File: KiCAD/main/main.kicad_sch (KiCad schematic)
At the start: 42 parts, among them J1 USB_C_Receptacle_USB2.0_14P, J2 Conn_Coaxial, SW1 SW_SPDT, SW2 SW_Push, SW3 SW_Push, U1 SX1262IMLTRT, U2 TP4056-42-ESOP8, U3 TLV75533PDRV, U4 ESP32-S3-MINI-1, U5 BGS12WN6E6327

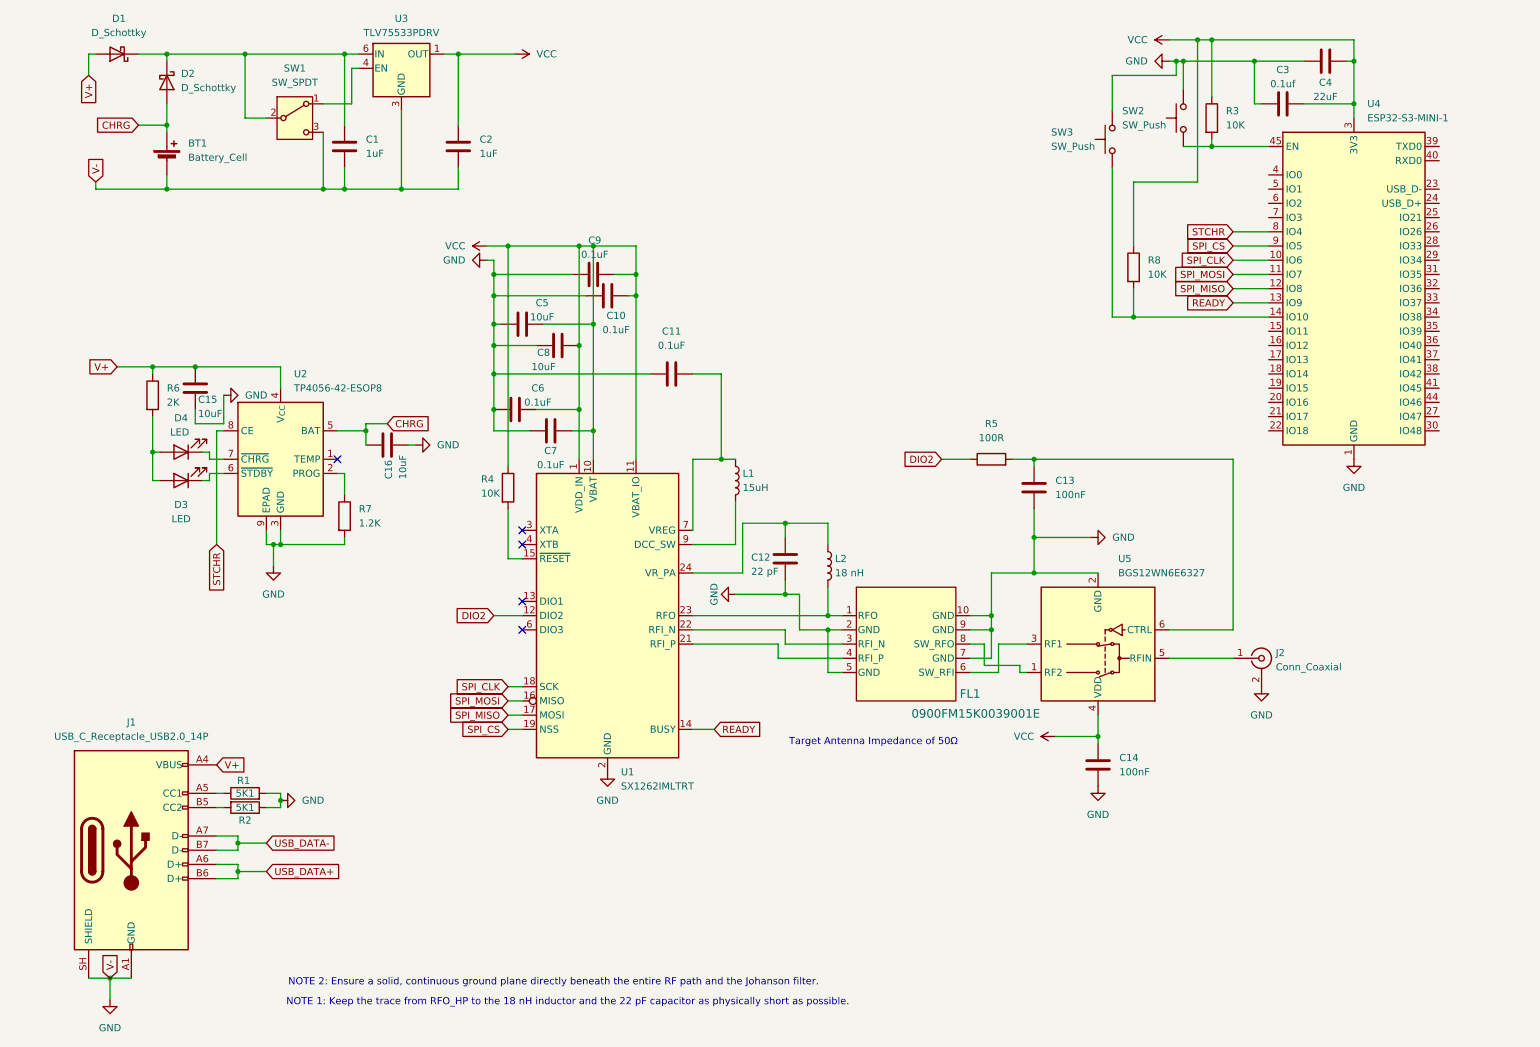
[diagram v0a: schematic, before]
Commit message: started repo and creation
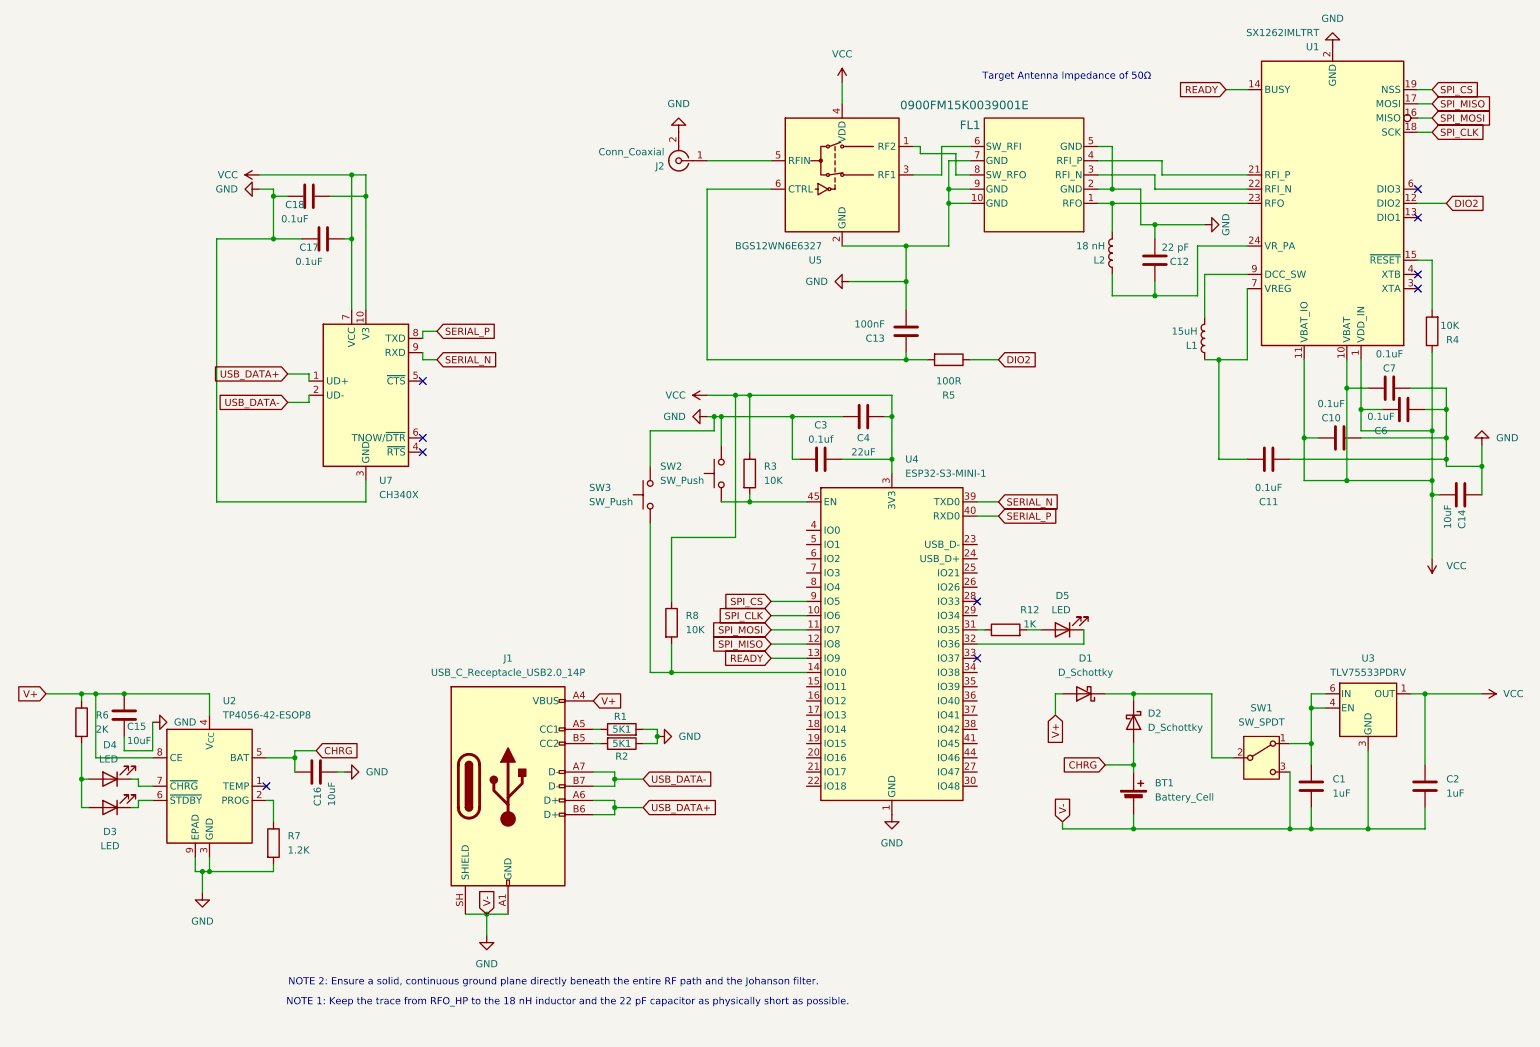
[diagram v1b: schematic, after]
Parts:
- removed C5, C8: 10uF, Capacitor_SMD:C_01005_0402Metric, symbol Device:C
- removed C9: 0.1uF, Capacitor_SMD:C_01005_0402Metric, symbol Device:C
- added C17, C18: 0.1uF, Capacitor_SMD:C_01005_0402Metric, symbol Device:C
- added D5: LED, LED_SMD:LED_0402_1005Metric, symbol Device:LED
- added R12: 1K, Resistor_SMD:R_01005_0402Metric, symbol Device:R
- added U7: CH340X, Package_SO:MSOP-10_3x3mm_P0.5mm, symbol Interface_USB:CH340X
- BT1: footprint Battery:BatteryHolder_MPD_BK-18650-PC2 -> Connector_JST:JST_PH_S2B-PH-K_1x02_P2.00mm_Horizontal
- C14: value 100nF -> 10uF
- R1, R2: footprint (none) -> Resistor_SMD:R_01005_0402Metric
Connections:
- net GND: now also C14.1, C17.1, C18.1, U7.3 (GND); no longer C14.2
- net USB_DATA+: now also U7.1 (UD+)
- net USB_DATA-: now also U7.2 (UD-)
- net V+: now also U2.8 (CE)
- net VCC: now also C14.2, C17.2, C18.2, U7.10 (V3), U7.7 (VCC); no longer C14.1
- net at U4.31 (IO35): now also R12.1
- net at U4.32 (IO36): now also D5.1 (K)
- net SERIAL_N: now reaches U4.39 (TXD0)
- net SERIAL_N: now also U7.9 (RXD)
- net SERIAL_P: now reaches U4.40 (RXD0)
- net SERIAL_P: now also U7.8 (TXD)
- net at D1.1 (K), D2.1 (K), SW1.2 (B): no longer C1.2, U3.6 (IN)
- net at SW1.1 (A), U3.4 (EN): now also C1.2, U3.6 (IN)
- net STCHR: no longer names the net of U4.8 (IO4)
- net STCHR: no longer U2.8 (CE)
- new net: D5.2 (A), R12.2
- no-connect marks 5 -> 10
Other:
- moved on the sheet: BT1, C1, C10, C11, C12, C13, C15, C16, C2, C3, C4, C6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

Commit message: rev 2!
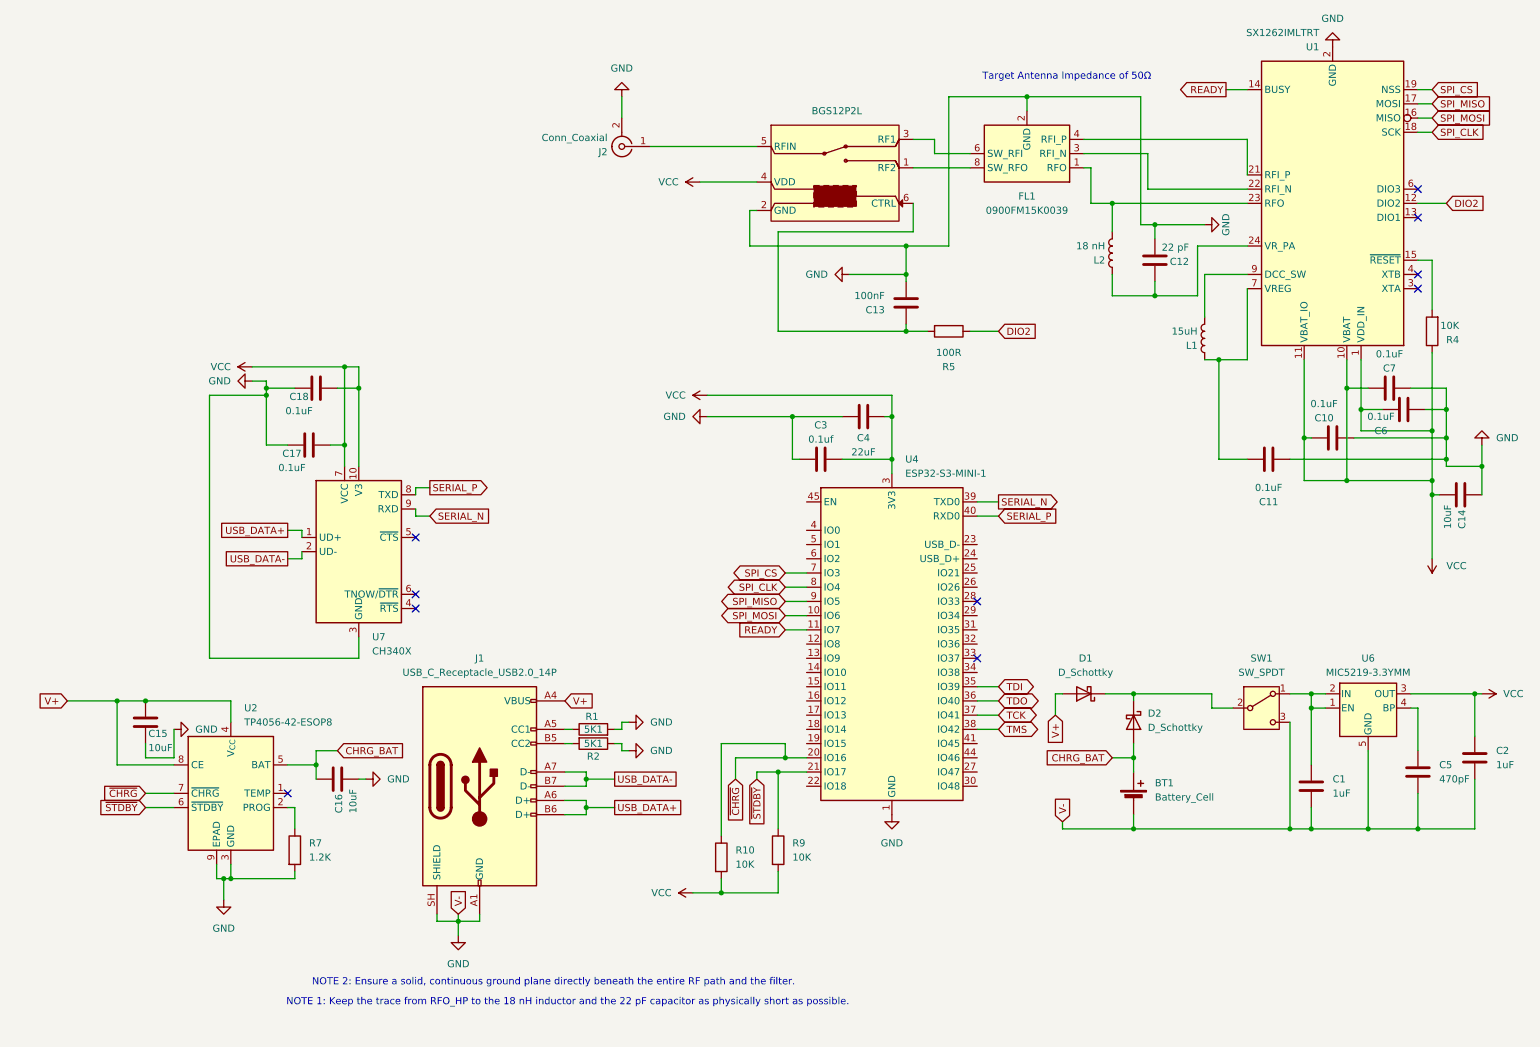
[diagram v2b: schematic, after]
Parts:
- removed D3, D4, D5: LED, LED_SMD:LED_0402_1005Metric, symbol Device:LED
- removed FL1: 0900FM15K0039001E, customlib:0900FM15K0039001E_JOT-L, symbol 2026-07-02_21-18-09:0900FM15K0039001E
- removed R12: 1K, Resistor_SMD:R_01005_0402Metric, symbol Device:R
- removed R3, R8: 10K, Resistor_SMD:R_01005_0402Metric, symbol Device:R
- removed R6: 2K, Resistor_SMD:R_01005_0402Metric, symbol Device:R
- removed SW2: SW_Push, Button_Switch_SMD:SW_SPST_PTS810, symbol Switch:SW_Push
- removed SW3: SW_Push, Button_Switch_SMD:SW_SPST_PTS645Sx43SMTR92, symbol Switch:SW_Push
- removed U3: TLV75533PDRV, Package_SON:WSON-6-1EP_2x2mm_P0.65mm_EP1x1.6mm, symbol Regulator_Linear:TLV75533PDRV
- removed U5: BGS12WN6E6327, Package_LGA:Infineon_PG-TSNP-6-10_0.7x1.1mm_0.7x1.1mm_P0.4mm, symbol RF_Switch:BGS12WN6E6327
- added C5: 470pF, Capacitor_SMD:C_0603_1608Metric, symbol Device:C
- added FL1: 0900FM15K0039, RF_Converter:Balun_Johanson_0900FM15K0039, symbol Filter:0900FM15K0039
- added R10, R9: 10K, Resistor_SMD:R_0603_1608Metric, symbol Device:R
- added U3: BGS12P2L, Package_LGA:Infineon_PG-TSNP-6-10_0.7x1.1mm_0.7x1.1mm_P0.4mm, symbol Personal:BGS12P2L
- added U6: MIC5219-3.3YMM, Package_SO:MSOP-8_3x3mm_P0.65mm, symbol Regulator_Linear:MIC5219-3.3YMM
- BT1: LCSC Part # (none) -> C265094
- C1, C2: footprint Capacitor_SMD:C_01005_0402Metric -> Capacitor_SMD:C_0603_1608Metric; LCSC Part # (none) -> C15849
- C10, C11, C13, C3, C6, C7: footprint Capacitor_SMD:C_01005_0402Metric -> Capacitor_SMD:C_0402_1005Metric; LCSC Part # (none) -> C1525
- C12: footprint Capacitor_SMD:C_01005_0402Metric -> Capacitor_SMD:C_0603_1608Metric; LCSC Part # (none) -> C1653
- C14, C15, C16: footprint Capacitor_SMD:C_01005_0402Metric -> Capacitor_SMD:C_0603_1608Metric; LCSC Part # (none) -> C19702
- C17, C18: footprint Capacitor_SMD:C_01005_0402Metric -> Capacitor_SMD:C_0402_1005Metric
- C4: footprint Capacitor_SMD:C_01005_0402Metric -> Capacitor_SMD:C_0805_2012Metric; LCSC Part # (none) -> C45783
- D1, D2: footprint Diode_SMD:D_01005_0402Metric -> Diode_SMD:D_SOD-323; LCSC Part # (none) -> C191023
- J1: LCSC Part # (none) -> C2765186
- J2: LCSC Part # (none) -> C3039673
- L1: footprint Inductor_SMD:L_01005_0402Metric -> Inductor_SMD:L_0805_2012Metric; LCSC Part # (none) -> C383402
- L2: footprint Inductor_SMD:L_01005_0402Metric -> Inductor_SMD:L_0603_1608Metric; LCSC Part # (none) -> C19721138
- R1, R2: footprint Resistor_SMD:R_01005_0402Metric -> Resistor_SMD:R_0603_1608Metric; LCSC Part # (none) -> C23186
- R4: footprint Resistor_SMD:R_01005_0402Metric -> Resistor_SMD:R_0603_1608Metric; LCSC Part # (none) -> C25804
- R5: footprint Resistor_SMD:R_01005_0402Metric -> Resistor_SMD:R_0402_1005Metric; LCSC Part # (none) -> C25076
- R7: footprint Resistor_SMD:R_01005_0402Metric -> Resistor_SMD:R_0603_1608Metric; LCSC Part # (none) -> C22765
- SW1: footprint Button_Switch_SMD:SW_SPDT_PCM12 -> customlib:SSSS810701; LCSC Part # (none) -> C97433
- U1: LCSC Part # (none) -> C191341
- U2: LCSC Part # (none) -> C16581
- U4: now left out of the parts list
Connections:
- net GND: now also C5.2, FL1.10 (GND), FL1.2 (GND), FL1.5 (GND), FL1.7 (GND), FL1.9 (GND), U3.2 (GND), U6.5 (GND), U6.6 (GND), U6.7 (GND), U6.8 (GND)
- net READY: now also U4.11 (IO7); no longer U4.13 (IO9)
- net SPI_CLK: now also U4.8 (IO4); no longer U4.10 (IO6)
- net SPI_CS: now also U4.7 (IO3); no longer U4.9 (IO5)
- net SPI_MISO: now also U4.9 (IO5); no longer U4.12 (IO8)
- net SPI_MOSI: now also U4.10 (IO6); no longer U4.11 (IO7)
- net VCC: now also R10.2, R9.2, U3.4 (VDD), U6.3 (OUT)
- net at J2.1 (In): now also U3.5 (RFIN)
- net at U1.21 (RFI_P): now also FL1.4 (RFI_P)
- net at U1.22 (RFI_N): now also FL1.3 (RFI_N)
- net at L2.2, U1.23 (RFO): now also FL1.1 (RFO)
- net ~{CHRG}: now reaches U4.20 (IO16)
- net ~{CHRG}: now also U2.7 (~{CHRG}), R10.1
- net ~{STDBY}: now reaches U4.21 (IO17)
- net ~{STDBY}: now also U2.6 (~{STDBY}), R9.1
- net TDI: now reaches U4.35 (IO39)
- net TDO: now reaches U4.36 (IO40)
- net TCK: now reaches U4.37 (IO41)
- net TMS: now reaches U4.38 (IO42)
- net at C1.2, SW1.1 (A): now also U6.1 (EN), U6.2 (IN)
- net at C13.1, R5.2: now also U3.6 (CTRL)
- net CHRG renamed CHRG_BAT
- new net: FL1.8 (SW_RFO), U3.1 (RF2)
- new net: FL1.6 (SW_RFI), U3.3 (RF1)
- new net: C5.1, U6.4 (BP)
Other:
- note added: "NOTE 2: Ensure a solid, continuous ground plane directly beneath the entire RF path and the filter."
- note removed: "NOTE 2: Ensure a solid, continuous ground plane directly beneath the entire RF path and the Johanson filter."
- moved on the sheet: C10, C13, C15, C16, C17, C18, C2, J1, J2, R1, R2, R5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
